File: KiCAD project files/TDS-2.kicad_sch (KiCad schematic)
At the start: 23 parts, among them J1 Barrel_Jack_MountingPin, J2 Conn_01x03_Pin, J3 Conn_01x03_Pin, J4 Conn_01x03_Pin, J5 SN49B14B, J6 SN49B14B, U1 TL072

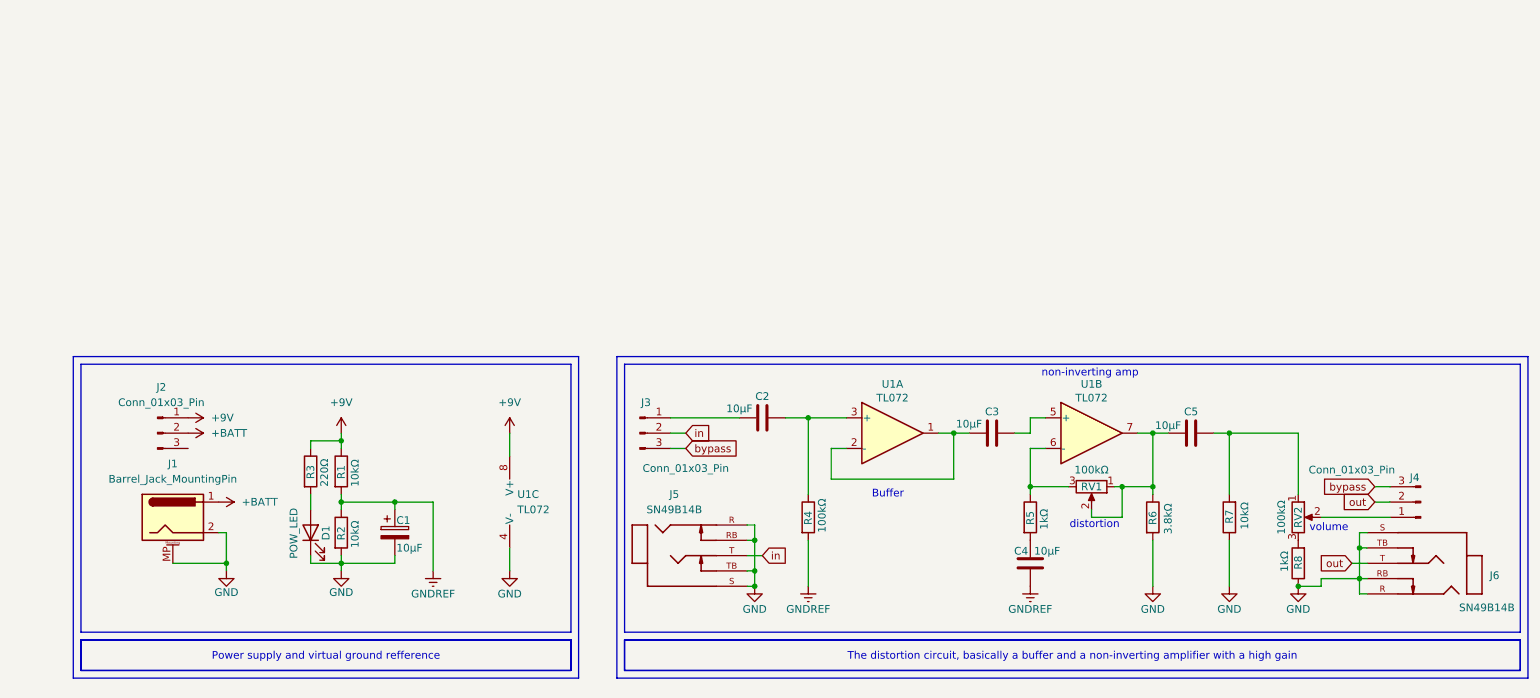
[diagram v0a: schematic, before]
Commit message: Update
Updated the schematic, idk about the photos tho
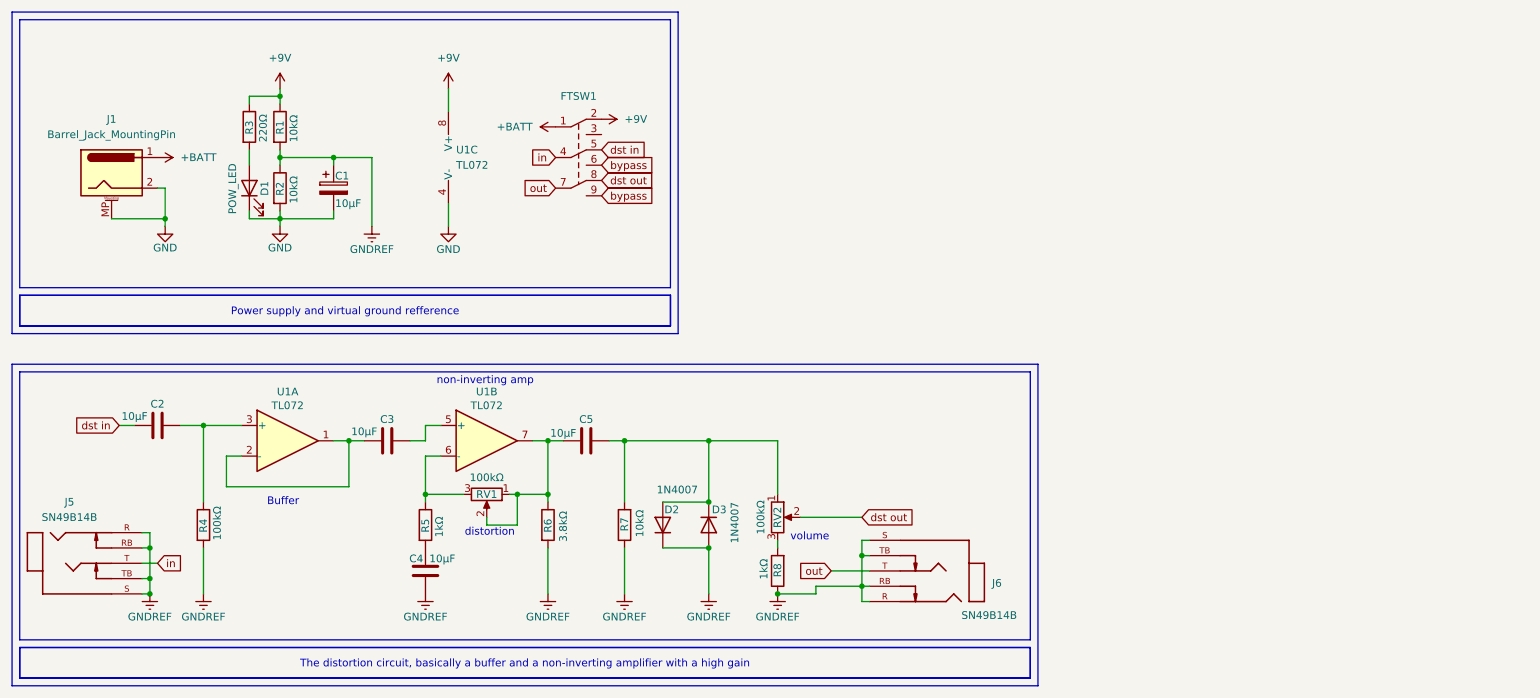
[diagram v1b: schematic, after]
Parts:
- removed J2, J3, J4: Conn_01x03_Pin, Connector_PinHeader_2.54mm:PinHeader_1x03_P2.54mm_Vertical, symbol Connector:Conn_01x03_Pin
- added D2, D3: 1N4007, Diode_THT:D_DO-41_SOD81_P10.16mm_Horizontal, symbol Diode:1N4007
- added FTSW1: ~, Library:3PDT Footswitch, symbol footswitch:3PDT_Footswitch
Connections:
- net +9V: now also FTSW1.2
- net +BATT: now also FTSW1.1
- net GND: no longer J5.R, J5.RB, J5.S, J5.TB, J6.R, J6.RB, J6.S, J6.TB, R6.2, R7.1, R8.1
- net GNDREF: now also J5.R, J5.RB, J5.S, J5.TB, J6.R, J6.RB, J6.S, J6.TB, R6.2, R7.1, R8.1, D2.1 (K), D3.2 (A)
- net bypass: now also FTSW1.6, FTSW1.9
- net in: now also FTSW1.4
- net out: now also FTSW1.7
- net dst in: now reaches C2.1
- net dst in: now also FTSW1.5
- net at C5.2, R7.2, RV2.1: now also D2.2 (A), D3.1 (K)
- net dst out: now reaches RV2.2
- net dst out: now also FTSW1.8
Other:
- moved on the sheet: C1, C2, C3, C4, C5, D1, J1, J5, J6, R1, R2, R3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
